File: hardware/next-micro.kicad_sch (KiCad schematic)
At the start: 25 parts, among them J1 USB_C_Receptacle_USB2.0, J2 Conn_01x13, J3 Conn_01x05, J4 Conn_01x13, SW1 RESET, U1 ATmega32U4-M, U2 RT9013-33GB, Y1 8MHz

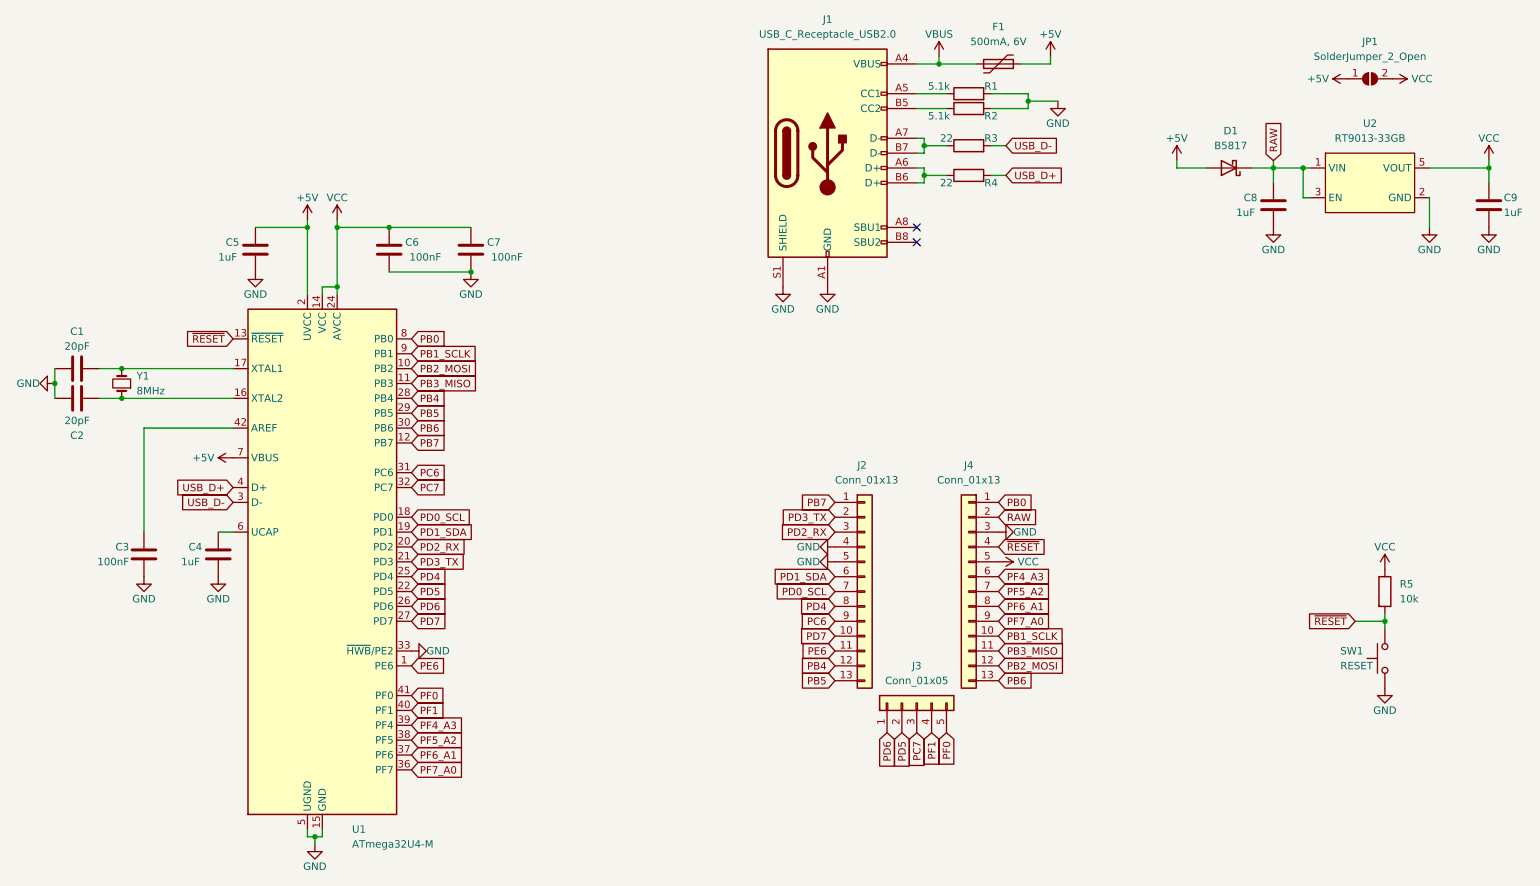
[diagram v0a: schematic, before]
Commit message: Add PCBA files and move files
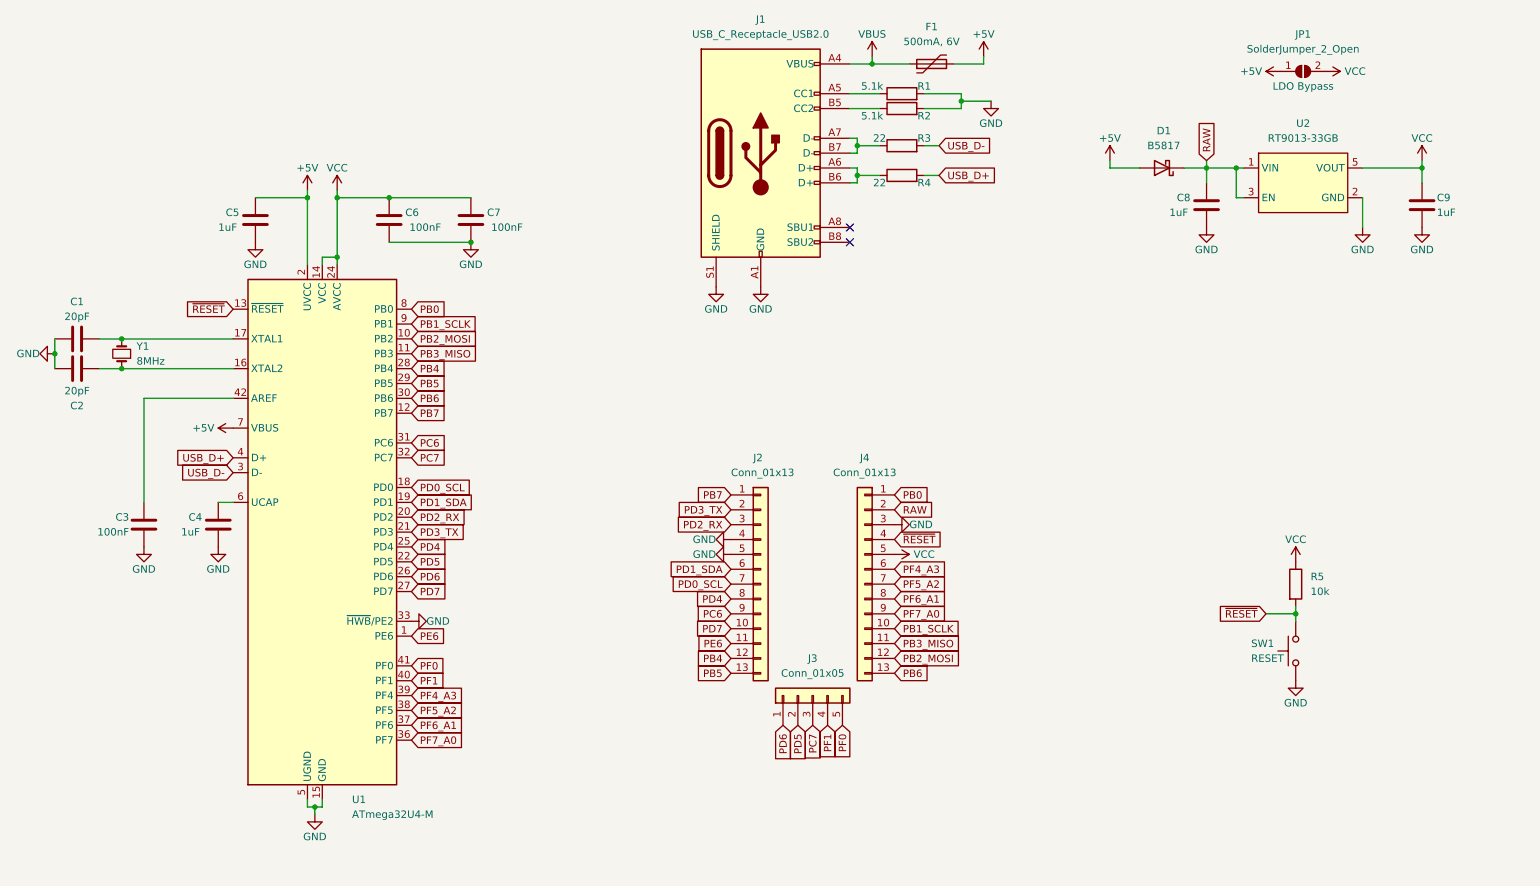
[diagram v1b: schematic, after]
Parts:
- J1: footprint rp-micro:USB Type-C Mid-Mount Receptacle 16P -> next_micro:USB Type-C Mid-Mount Receptacle 16P
- JP1: Note (none) -> LDO Bypass
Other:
- title: (none) -> Next Micro
- moved on the sheet: C1, C2, C3, C4, C5, C6, C7, C8, C9, D1, F1, J1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
